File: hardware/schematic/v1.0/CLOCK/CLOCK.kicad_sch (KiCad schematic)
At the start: 23 parts, among them J1 Conn_Coaxial, J2 Conn_Coaxial, J3 Conn_Coaxial, J4 Conn_Coaxial, J5 Conn_Coaxial, U1 LMK5B12204, U2 LMK1C1102

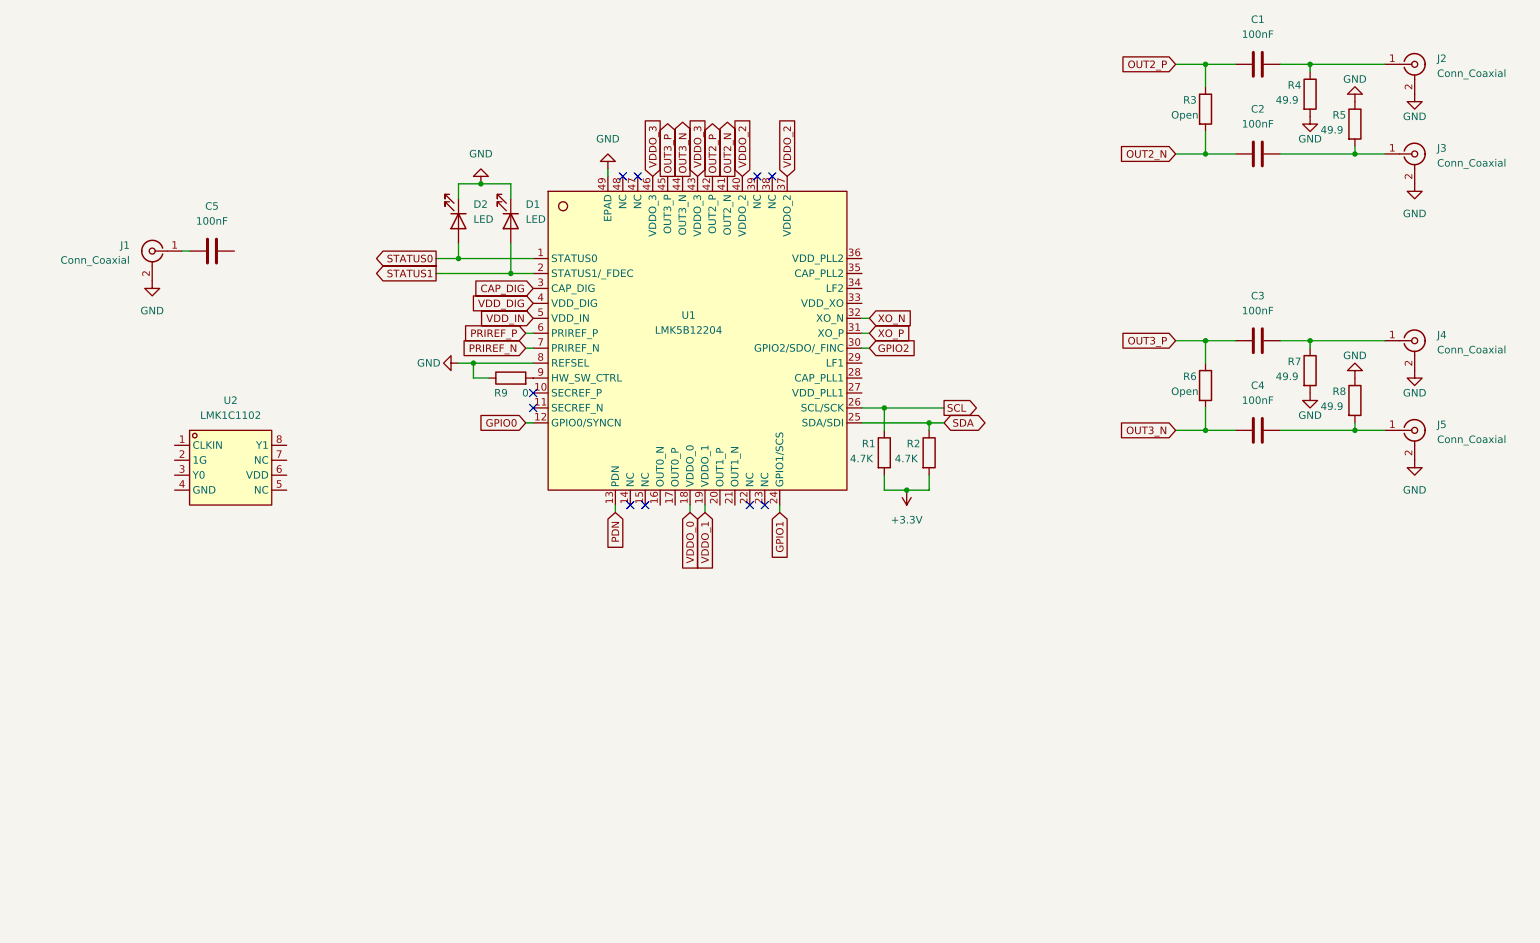
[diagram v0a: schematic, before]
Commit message: sch commit
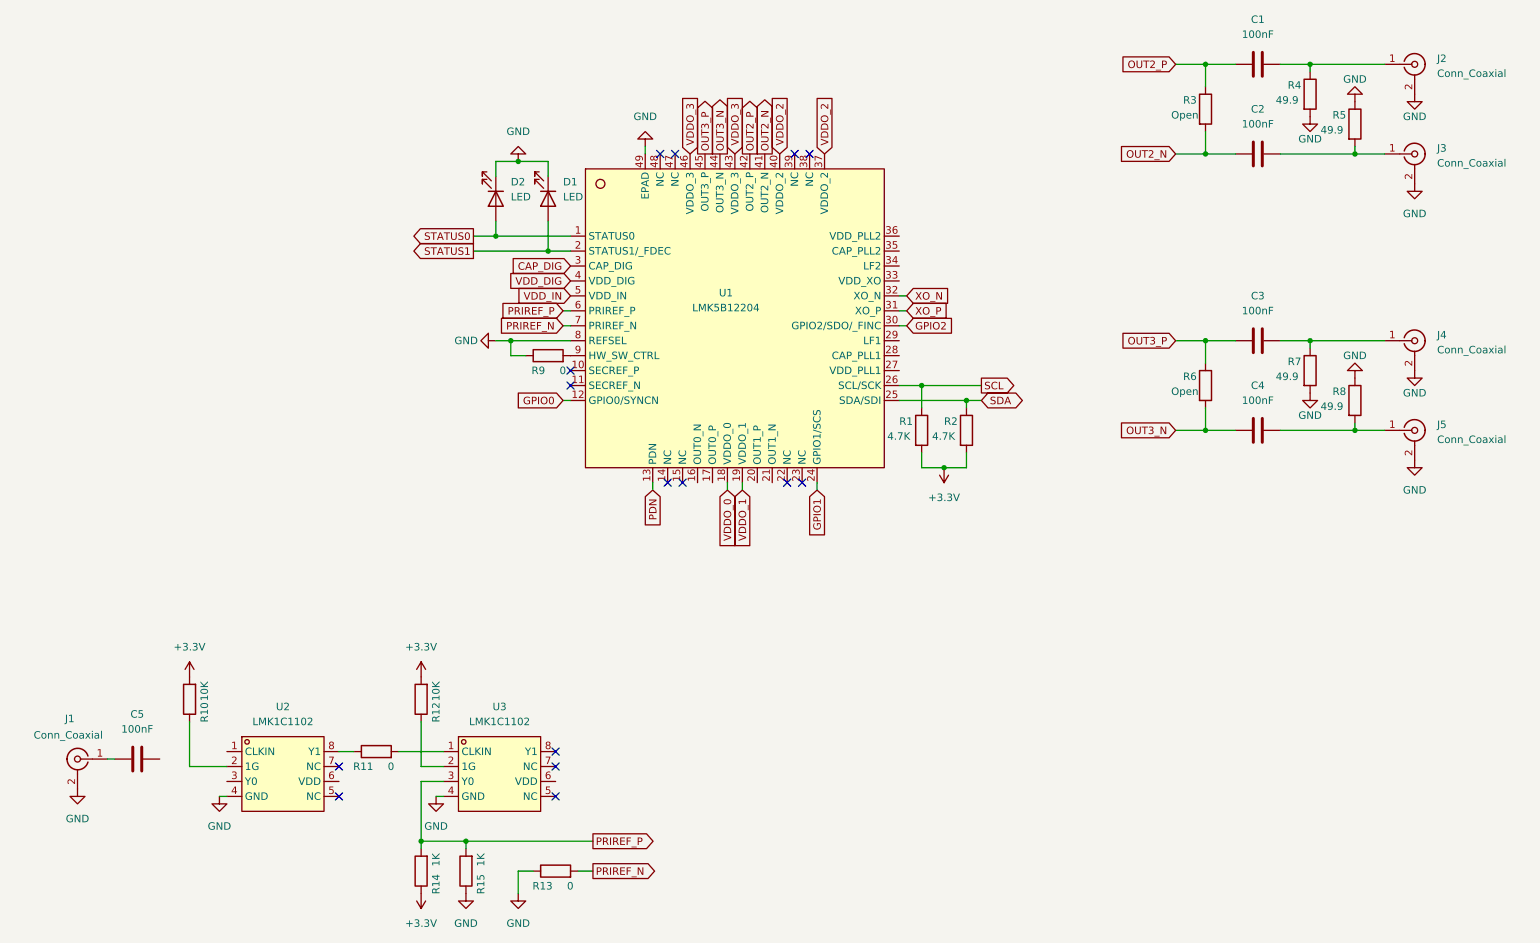
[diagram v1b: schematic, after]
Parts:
- added R10, R12: 10K, Resistor_SMD:R_0402_1005Metric, symbol Device:R
- added R11, R13: 0, Resistor_SMD:R_0402_1005Metric, symbol Device:R
- added R14, R15: 1K, Resistor_SMD:R_0402_1005Metric, symbol Device:R
- added U3: LMK1C1102, Package_SON:WSON-8-1EP_2x2mm_P0.5mm_EP0.9x1.6mm, symbol Counter:LMK1C1102
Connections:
- net +3.3V: now also R10.2, R12.2, R14.1
- net GND: now also U2.4 (GND), R13.1, R15.1, U3.4 (GND)
- net PRIREF_N: now also R13.2
- net PRIREF_P: now also R14.2, R15.2, U3.3 (Y0)
- net at U2.2 (1G): now also R10.1
- net at U2.8 (Y1): now also R11.1
- new net: R12.1, U3.2 (1G)
- new net: R11.2, U3.1 (CLKIN)
- no-connect marks 10 -> 15
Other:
- moved on the sheet: C5, D1, D2, J1, R1, R2, R9, U1, U2
